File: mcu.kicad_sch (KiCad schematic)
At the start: 16 parts, among them J1 Conn_ARM_SWD_TagConnect_TC2030, U2 STM32L053R8Tx

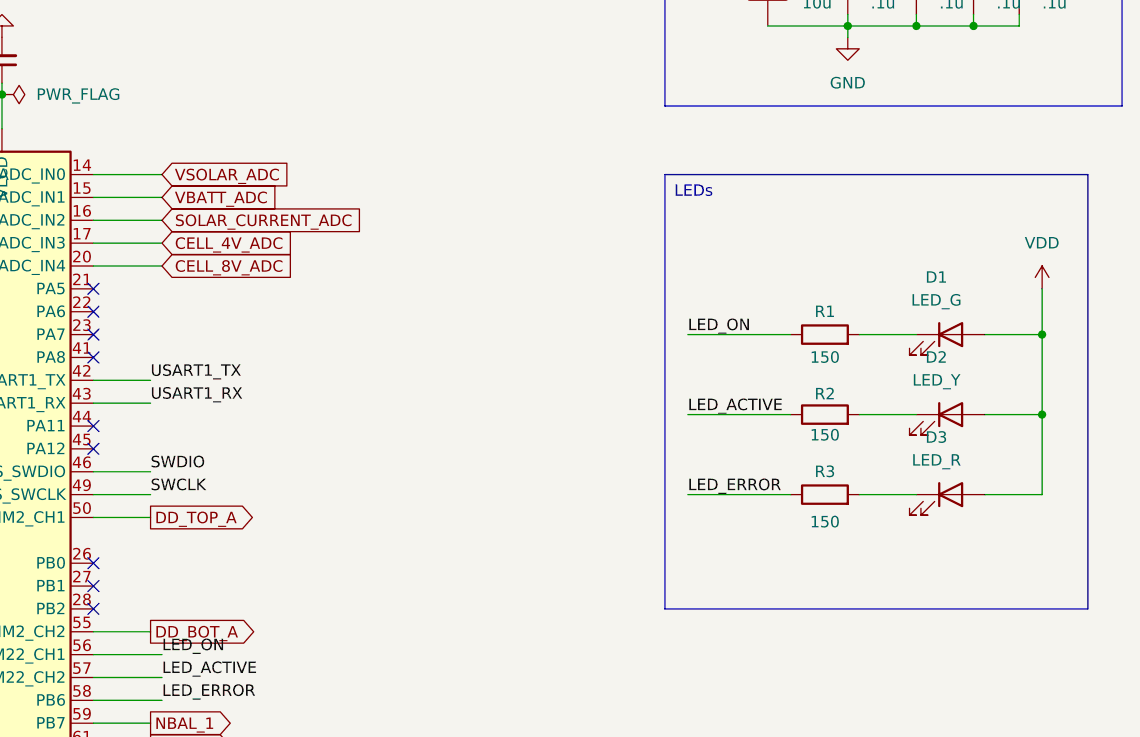
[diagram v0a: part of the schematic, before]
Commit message: New design and layout
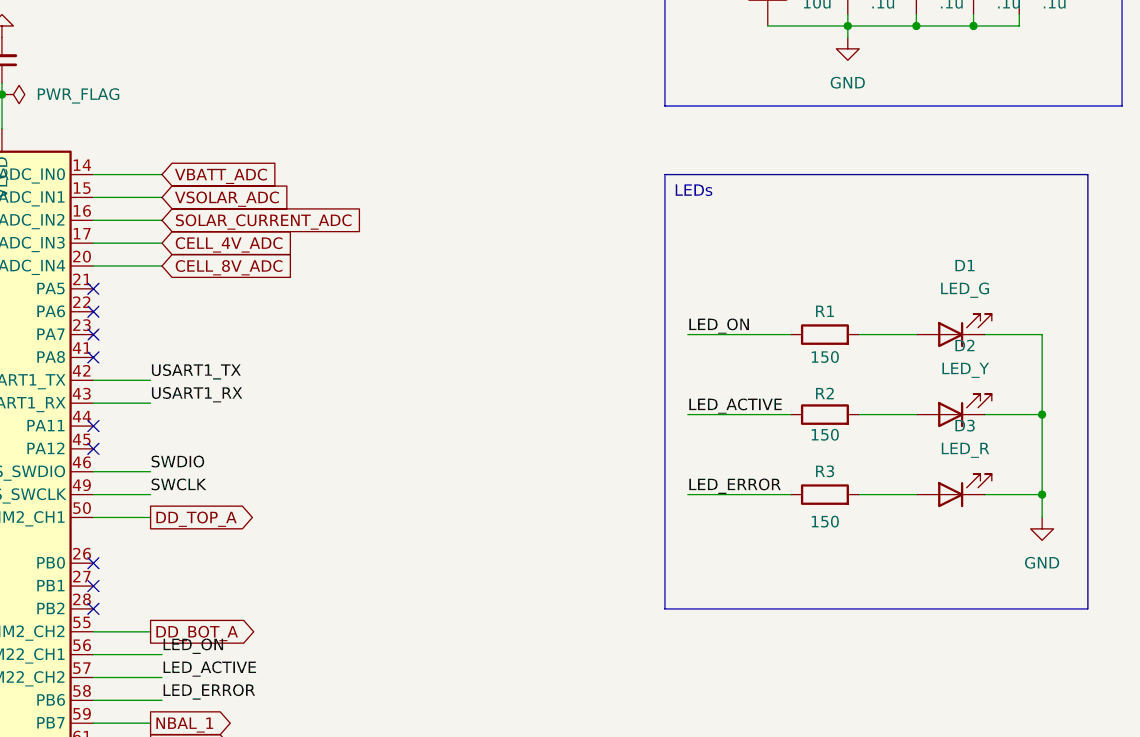
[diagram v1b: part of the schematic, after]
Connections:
- net GND: now also D1.1 (K), D2.1 (K), D3.1 (K)
- net VBATT_ADC: now also U2.14 (PA0); no longer U2.15 (PA1)
- net VDD: no longer D1.2 (A), D2.2 (A), D3.2 (A)
- net VSOLAR_ADC: now also U2.15 (PA1); no longer U2.14 (PA0)
- net at R3.2: now also D3.2 (A); no longer D3.1 (K)
- net at R1.2: now also D1.2 (A); no longer D1.1 (K)
- net at R2.2: now also D2.2 (A); no longer D2.1 (K)
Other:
- moved on the sheet: D1, D2, D3
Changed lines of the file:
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@@
+	)
+	(junction
+		(at 264.16 86.36)
+		(diameter 0)
+		(color 0 0 0 0)
 	)
 	(junction
@@
 	)
 	(junction
-		(at 264.16 68.58)
-		(diameter 0)
-		(color 0 0 0 0)
-	)
-	(junction
 		(at 250.19 26.67)
 		(diameter 0)
@@
 	(wire
 		(pts
+			(xy 264.16 88.9) (xy 264.16 86.36)
+		)
+		(stroke
+			(width 0)
+			(type default)
+		)
+	)
+	(wire
+		(pts
 			(xy 158.75 111.76) (xy 165.1 111.76)
 		)
@@
 		(pts
 			(xy 140.97 45.72) (xy 140.97 43.18)
-		)
-		(stroke
-			(width 0)
-			(type default)
-		)
-	)
-	(wire
-		(pts
-			(xy 264.16 63.5) (xy 264.16 68.58)
 		)
 		(stroke
@@
 	(global_label "VBATT_ADC"
 		(shape input)
-		(at 166.37 53.34 0)
+		(at 166.37 50.8 0)
 		(fields_autoplaced yes)
 		(effects
@@
 		)
 		(property "Intersheetrefs" "${INTERSHEET_REFS}"
-			(at 179.3338 53.34 0)
+			(at 179.3338 50.8 0)
 			(effects
 				(font
@@
 	(global_label "VSOLAR_ADC"
 		(shape input)
-		(at 166.37 50.8 0)
+		(at 166.37 53.34 0)
 		(fields_autoplaced yes)
 		(effects
@@
 		)
 		(property "Intersheetrefs" "${INTERSHEET_REFS}"
-			(at 180.9667 50.8 0)
+			(at 180.9667 53.34 0)
 			(effects
 				(font
@@
 	(symbol
 		(lib_id "Device:LED")
-		(at 254 86.36 0)
+		(at 254 86.36 180)
 		(unit 1)
 		(exclude_from_sim no)
@@
 		(fields_autoplaced yes)
 		(property "Reference" "D3"
-			(at 252.4125 80.01 0)
+			(at 255.5875 78.74 0)
 			(effects
 				(font
@@
 		)
 		(property "Value" "LED_R"
-			(at 252.4125 82.55 0)
+			(at 255.5875 81.28 0)
 			(effects
 				(font
@@
 	(symbol
 		(lib_id "Device:LED")
-		(at 254 68.58 0)
+		(at 254 68.58 180)
 		(unit 1)
 		(exclude_from_sim no)
@@
 		(fields_autoplaced yes)
 		(property "Reference" "D1"
-			(at 252.4125 62.23 0)
+			(at 255.5875 60.96 0)
 			(effects
 				(font
@@
 		)
 		(property "Value" "LED_G"
-			(at 252.4125 64.77 0)
+			(at 255.5875 63.5 0)
 			(effects
 				(font
@@
 	)
 	(symbol
+		(lib_id "power:GND")
+		(at 264.16 88.9 0)
+		(unit 1)
+		(exclude_from_sim no)
+		(in_bom yes)
+		(on_board yes)
+		(dnp no)
+		(fields_autoplaced yes)
+		(property "Reference" "#PWR015"
+			(at 264.16 95.25 0)
+			(effects
+				(font
+					(size 1.27 1.27)
+				)
+				(hide yes)
+			)
+		)
+		(property "Value" "GND"
+			(at 264.16 93.98 0)
+			(effects
+				(font
+					(size 1.27 1.27)
+				)
+			)
+		)
+		(property "Footprint" ""
+			(at 264.16 88.9 0)
+			(effects
+				(font
+					(size 1.27 1.27)
+				)
+				(hide yes)
+			)
+		)
+		(property "Datasheet" ""
+			(at 264.16 88.9 0)
+			(effects
+				(font
+					(size 1.27 1.27)
+				)
+				(hide yes)
+			)
+		)
+		(property "Description" "Power symbol creates a global label with name \"GND\" , ground"
+			(at 264.16 88.9 0)
+			(effects
+				(font
+					(size 1.27 1.27)
+				)
+				(hide yes)
+			)
+		)
+		(pin "1"
+		)
+		(instances
+			(project "JPBms2"
+				(path "/d86e471c-a8be-422d-a5d1-5a4699b7b766/852788cb-2266-4d4a-865c-a7e0873e4190"
+					(reference "#PWR015")
+					(unit 1)
+				)
+			)
+		)
+	)
+	(symbol
 		(lib_id "Device:C_Small")
 		(at 148.59 38.1 180)
@@
 	)
 	(symbol
-		(lib_id "power:VDD")
-		(at 264.16 63.5 0)
+		(lib_id "Device:LED")
+		(at 254 77.47 180)
 		(unit 1)
 		(exclude_from_sim no)
@@
 		(on_board yes)
 		(dnp no)
-		(property "Reference" "#PWR015"
-			(at 264.16 67.31 0)
-			(effects
-				(font
-					(size 1.27 1.27)
-				)
-				(hide yes)
-			)
-		)
-		(property "Value" "VDD"
-			(at 264.16 58.42 0)
-			(effects
-				(font
-					(size 1.27 1.27)
-				)
-			)
-		)
-		(property "Footprint" ""
-			(at 264.16 63.5 0)
-			(effects
-				(font
-					(size 1.27 1.27)
-				)
-				(hide yes)
-			)
-		)
-		(property "Datasheet" ""
-			(at 264.16 63.5 0)
-			(effects
-				(font
-					(size 1.27 1.27)
-				)
-				(hide yes)
-			)
-		)
-		(property "Description" "Power symbol creates a global label with name \"VDD\""
-			(at 264.16 63.5 0)
-			(effects
-				(font
-					(size 1.27 1.27)
-				)
-				(hide yes)
-			)
-		)
-		(pin "1"
-		)
-		(instances
-			(project "JPBms2"
-				(path "/d86e471c-a8be-422d-a5d1-5a4699b7b766/852788cb-2266-4d4a-865c-a7e0873e4190"
-					(reference "#PWR015")
-					(unit 1)
-				)
-			)
-		)
-	)
-	(symbol
-		(lib_id "Device:LED")
-		(at 254 77.47 0)
-		(unit 1)
-		(exclude_from_sim no)
-		(in_bom yes)
-		(on_board yes)
-		(dnp no)
 		(fields_autoplaced yes)
 		(property "Reference" "D2"
-			(at 252.4125 71.12 0)
+			(at 255.5875 69.85 0)
 			(effects
 				(font
@@
 		)
 		(property "Value" "LED_Y"
-			(at 252.4125 73.66 0)
-			(effects
-				(font
+			(at 255.5875 72.39 0)
+			(effects
+				(font
